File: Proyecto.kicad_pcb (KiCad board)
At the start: 2 copper layers, 135 x 90 mm, 46 parts, among them P1 CONN_01X03, P2 CONN_01X03, Q1 BC808-40, Q2 BC808-40, U1 MCP2515, U2 MCP2551-I/SN, U3 AMS1117, U4 ACS712, U5 ACS712

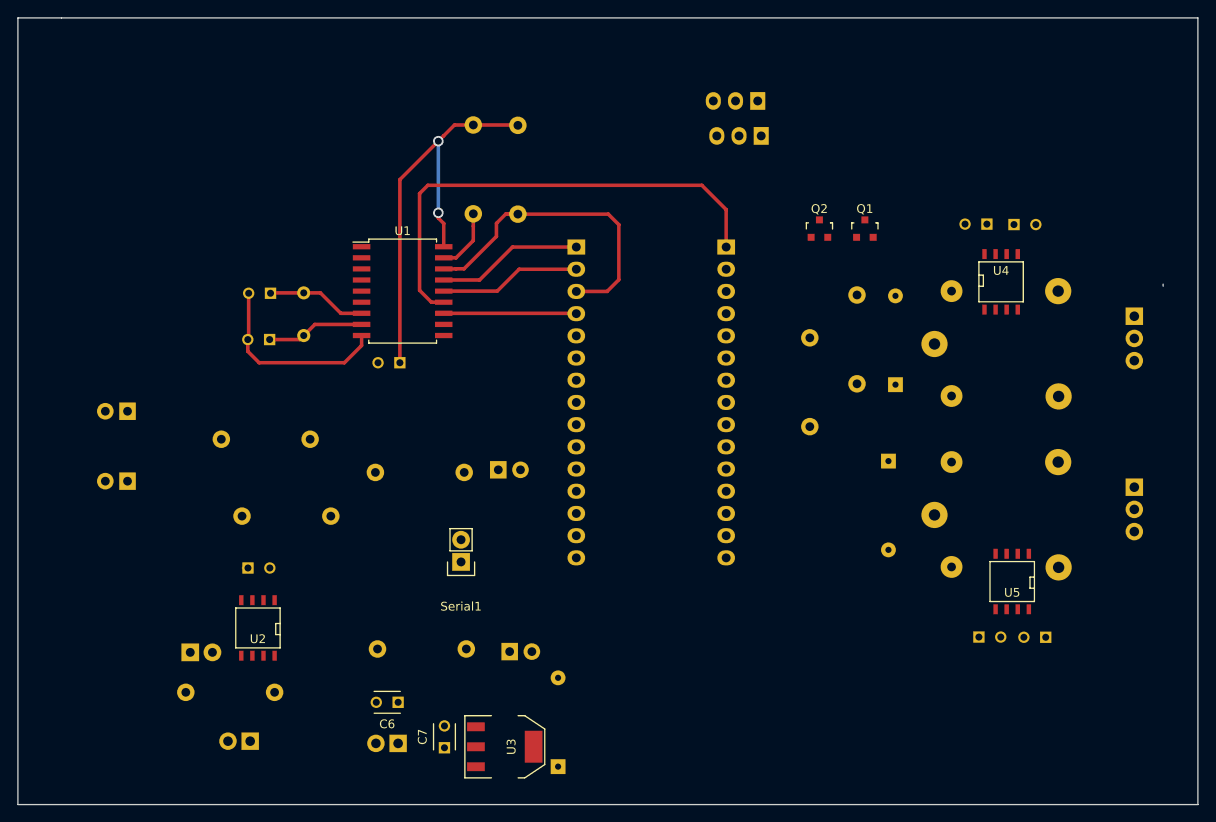
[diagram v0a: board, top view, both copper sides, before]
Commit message: fix terrena
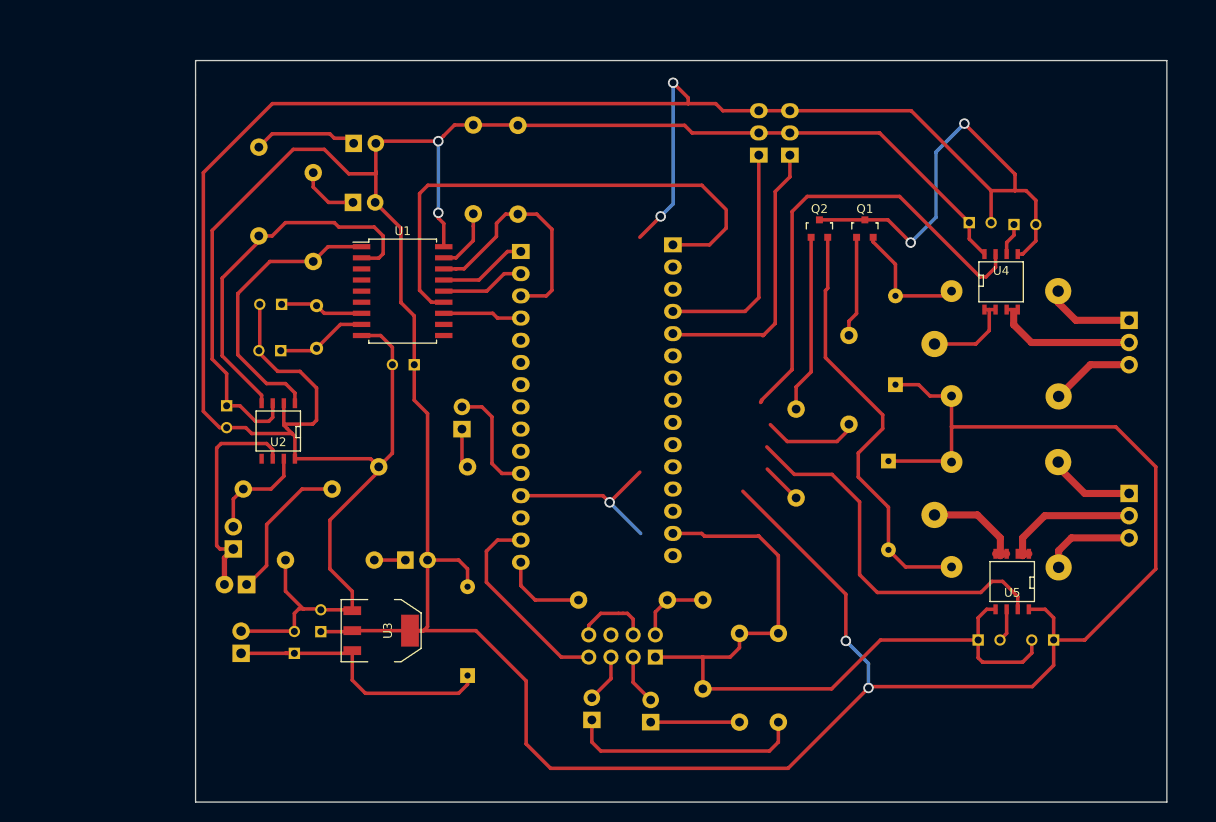
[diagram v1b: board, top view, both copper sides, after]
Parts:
- removed D4: LED 2, LEDs:LED-5MM
- removed LED_BLINK1: LED, LEDs:LED-5MM
- removed Serial1: CONN_01X02, Pin_Headers:Pin_Header_Straight_1x02
- added ESP8266: CONN_02X04, Pin_Headers:Pin_Header_Straight_2x04, B.Cu at (112.9, 108.1)
- added LED1: LED, LEDs:LED-5MM, B.Cu at (90.8, 82.0)
- added LED_Gp1: LED, LEDs:LED-5MM, B.Cu at (105.7, 115.3)
- added LED_Gp2: LED, LEDs:LED-5MM, B.Cu at (112.4, 115.6)
- added LED_Vcc1: LED, LEDs:LED-5MM, B.Cu at (84.3, 97.0)
- added R12: 1k, Resistors_ThroughHole:Resistor_Horizontal_RM10mm, B.Cu at (104.1, 101.6)
- added R13: 2k2, Resistors_ThroughHole:Resistor_Horizontal_RM10mm, B.Cu at (118.4, 101.6)
- added R6: 1k, Resistors_ThroughHole:Resistor_Horizontal_RM10mm, B.Cu at (122.6, 115.6)
- added R7: 1k, Resistors_ThroughHole:Resistor_Horizontal_RM10mm, B.Cu at (127.0, 115.6)
- C6, C7: moved to B.Cu
- moved C10 97.4 mm to (63.9, 79.4), turned to 270 degrees
- moved C4 91.5 mm to (148.8, 58.4)
- moved C3 81.2 mm to (158.5, 106.2)
- moved C11 67.5 mm to (85.3, 74.7)
- moved D_TX1 41.0 mm to (78.3, 56.1), turned to 0 degrees
- moved R8 40.1 mm to (73.8, 52.7), turned to 270 degrees
- moved D_RX1 40.1 mm to (78.4, 49.4), turned to 0 degrees
- moved R9 33.7 mm to (67.6, 49.8), turned to 270 degrees
- moved R5 23.5 mm to (65.8, 88.9), turned to 0 degrees
- moved U2 22.7 mm to (69.8, 82.3)
- moved CAN1 22.1 mm to (64.6, 95.8), turned to 90 degrees
- moved S0 20.7 mm to (65.5, 107.7), turned to 90 degrees
- moved C7 19.4 mm to (74.7, 105.2)
- moved U3 19.4 mm to (81.6, 105.1)
- moved D1 14.7 mm to (91.4, 110.2)
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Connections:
- PIN_L1 pad 12: Net-(PIN_L1-Pad12) -> GND
- PIN_L1 pad 14: /tx -> Net-(ESP8266-Pad7)
- PIN_L1 pad 15: /rx -> Net-(PIN_L1-Pad15)
- PIN_R1 pad 10: /R2 -> /AC2
- PIN_R1 pad 2: Net-(PIN_R1-Pad2) -> /3.3V
- PIN_R1 pad 8: /AC2 -> /AC1
- PIN_R1 pad 9: /AC1 -> /R2
- S0 pad 1: Net-(C6-Pad1) -> Net-(S0-Pad1)
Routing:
- net GND: track 22.2 -> 422.4 mm, vias 0 -> 5
- net +5V: track 49.9 -> 421.4 mm, vias 2 -> 4
- net (no net): track 141.5 -> 0.00 mm
- net /AC1: track 0.00 -> 53.1 mm
- net Net-(D3-Pad2): track 0.00 -> 49.2 mm
- net /AC2: track 0.00 -> 43.2 mm
- net Net-(R9-Pad2): track 1.52 -> 43.0 mm
- net Net-(R8-Pad2): track 0.00 -> 32.9 mm
- net pin23: track 0.00 -> 32.4 mm
- net Net-(C6-Pad1): track 0.00 -> 27.4 mm
- net Net-(LED_Gp1-Pad1): track 0.00 -> 27.0 mm
- net pin24: track 0.00 -> 26.8 mm
- net Net-(CAN1-Pad1): track 0.00 -> 25.7 mm
- net Net-(ESP8266-Pad7): track 0.00 -> 23.3 mm
- net Net-(Q2-Pad1): track 0.00 -> 20.4 mm
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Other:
- board size 135 x 90 mm -> 111.1 x 84.8 mm
